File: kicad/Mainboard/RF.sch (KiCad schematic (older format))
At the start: 97 parts, among them J7 Antenna, T1 AFT05MS004NT1, U5 HMC546MS8GETR

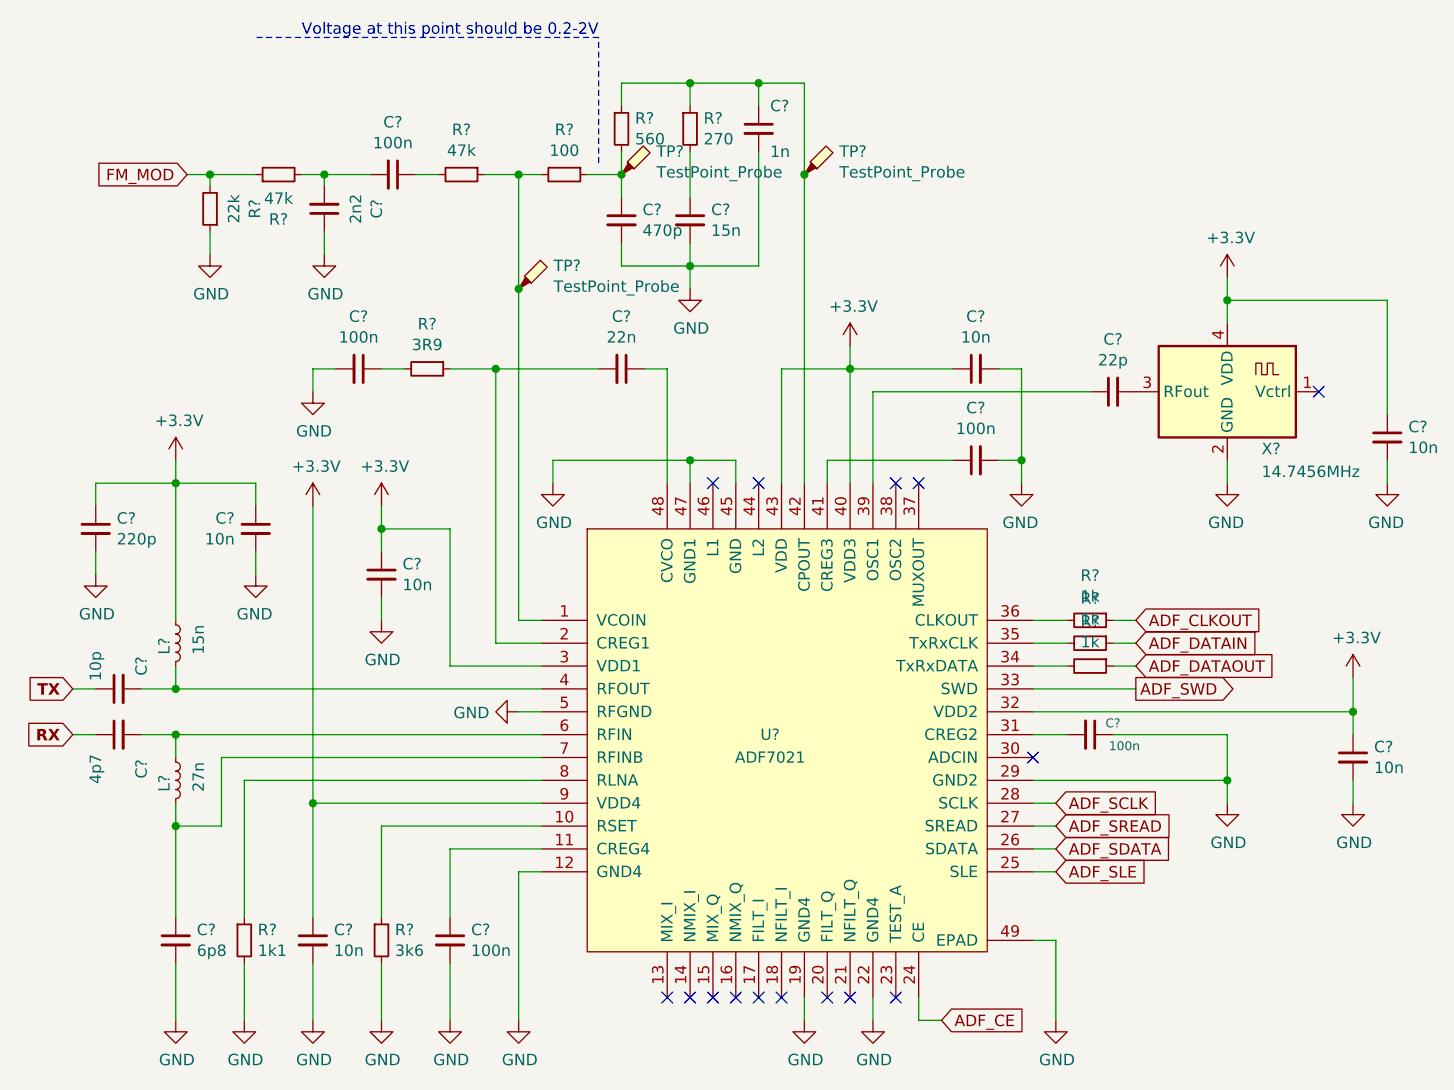
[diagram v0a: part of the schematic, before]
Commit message: Add files via upload
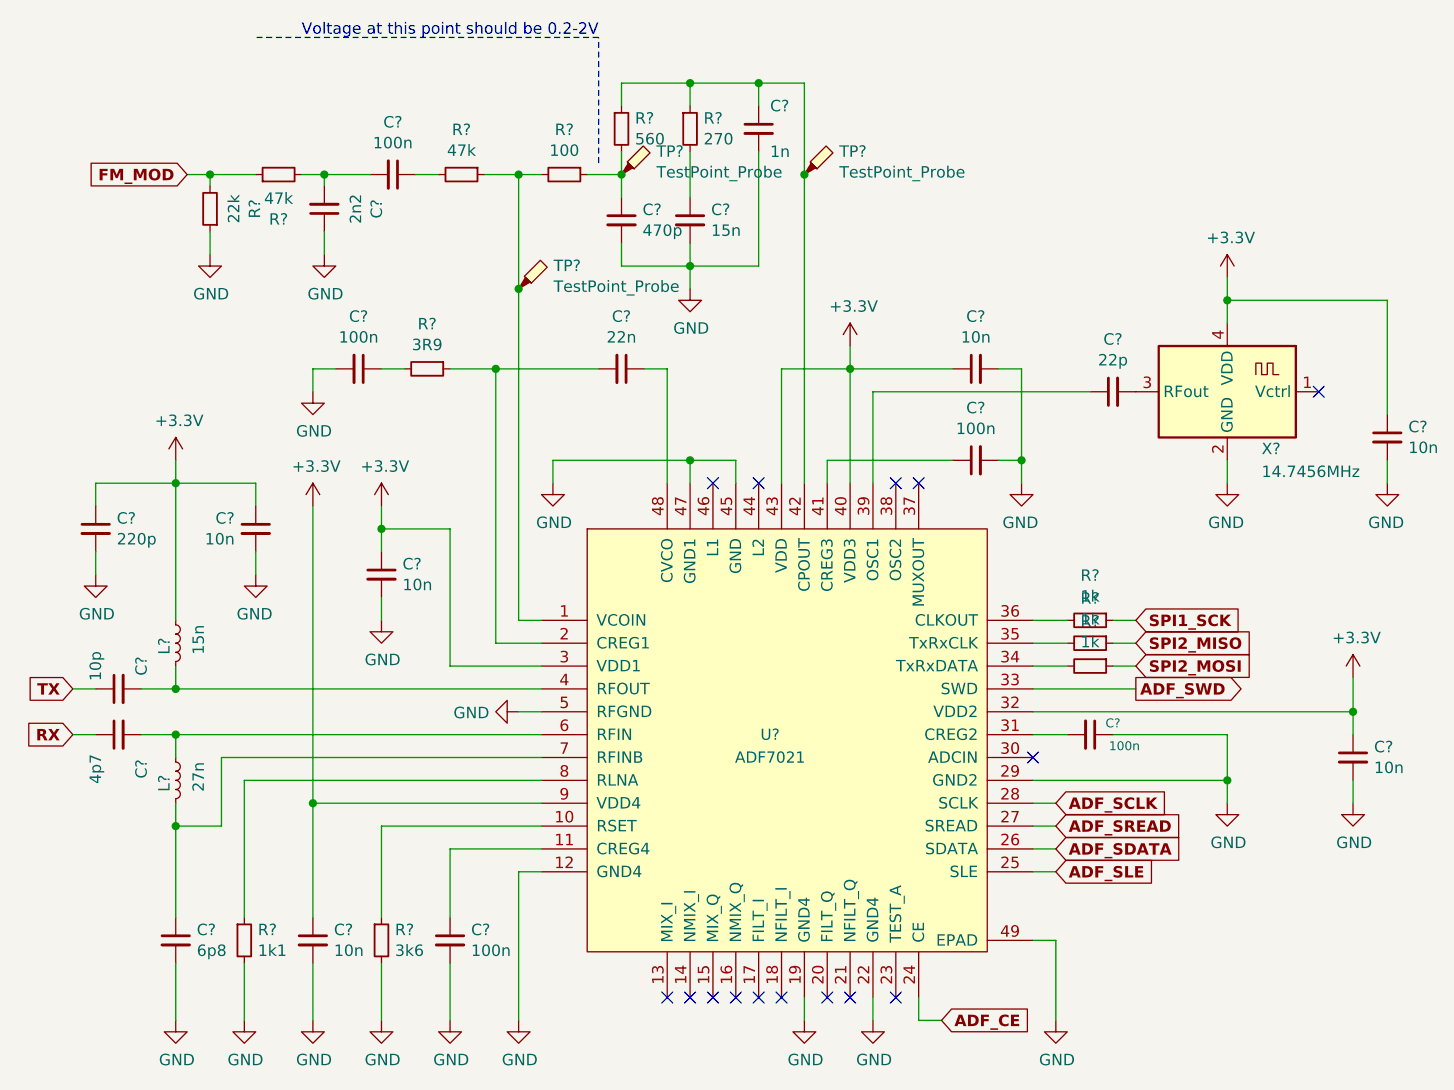
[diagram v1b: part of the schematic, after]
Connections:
- net ADF_CLKOUT renamed SPI1_SCK
- net ADF_DATAIN renamed SPI2_MISO
- net ADF_DATAOUT renamed SPI2_MOSI
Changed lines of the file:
@@
 Wire Wire Line
 	6600 8450 6700 8450
-Text GLabel 6700 8250 2    50   Input ~ 0
-ADF_CLKOUT
-Text GLabel 6700 8350 2    50   Input ~ 0
-ADF_DATAIN
-Text GLabel 6700 8450 2    50   Input ~ 0
-ADF_DATAOUT
 $Comp
 L Device:C_Small C?
@@
 Wire Wire Line
 	6250 9350 6350 9350
-Text GLabel 6350 9050 2    50   Input ~ 0
+Text GLabel 6350 9050 2    50   Input ~ 10
 ADF_SCLK
-Text GLabel 6350 9150 2    50   Input ~ 0
+Text GLabel 6350 9150 2    50   Input ~ 10
 ADF_SREAD
-Text GLabel 6350 9250 2    50   Input ~ 0
+Text GLabel 6350 9250 2    50   Input ~ 10
 ADF_SDATA
-Text GLabel 6350 9350 2    50   Input ~ 0
+Text GLabel 6350 9350 2    50   Input ~ 10
 ADF_SLE
 Wire Wire Line
@@
 Wire Wire Line
 	5750 10000 5850 10000
-Text GLabel 5850 10000 2    50   Input ~ 0
+Text GLabel 5850 10000 2    50   Input ~ 10
 ADF_CE
 NoConn ~ 5650 9900
@@
 Wire Wire Line
 	6250 8550 6700 8550
-Text GLabel 6700 8550 2    50   Output ~ 0
+Text GLabel 6700 8550 2    50   Output ~ 10
 ADF_SWD
 $Comp
@@
 Wire Wire Line
 	3650 6300 3550 6300
-Text GLabel 2550 6300 0    50   Input ~ 0
+Text GLabel 2550 6300 0    50   Input ~ 10
 FM_MOD
 Text Notes 4350 5700 2    50   ~ 0
@@
 Wire Wire Line
 	13300 5800 13600 5800
+Text GLabel 6700 8250 2    50   Input ~ 10
+SPI1_SCK
+Text GLabel 6700 8350 2    50   Input ~ 10
+SPI2_MISO
+Text GLabel 6700 8450 2    50   Input ~ 10
+SPI2_MOSI
 $EndSCHEMATC
